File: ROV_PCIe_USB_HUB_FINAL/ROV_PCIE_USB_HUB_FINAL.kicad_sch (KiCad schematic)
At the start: 13 parts, among them J1 USB_A_Stacked, J2 USB_A_Stacked, J3 USB_A_Stacked, J4 USB_A_Stacked, U1 UPD720202K8-7x1-BAA, U2 USB2514B_Bi, U3 USB2514B_Bi, U4 USB2514B_Bi, U5 USB2514B_Bi

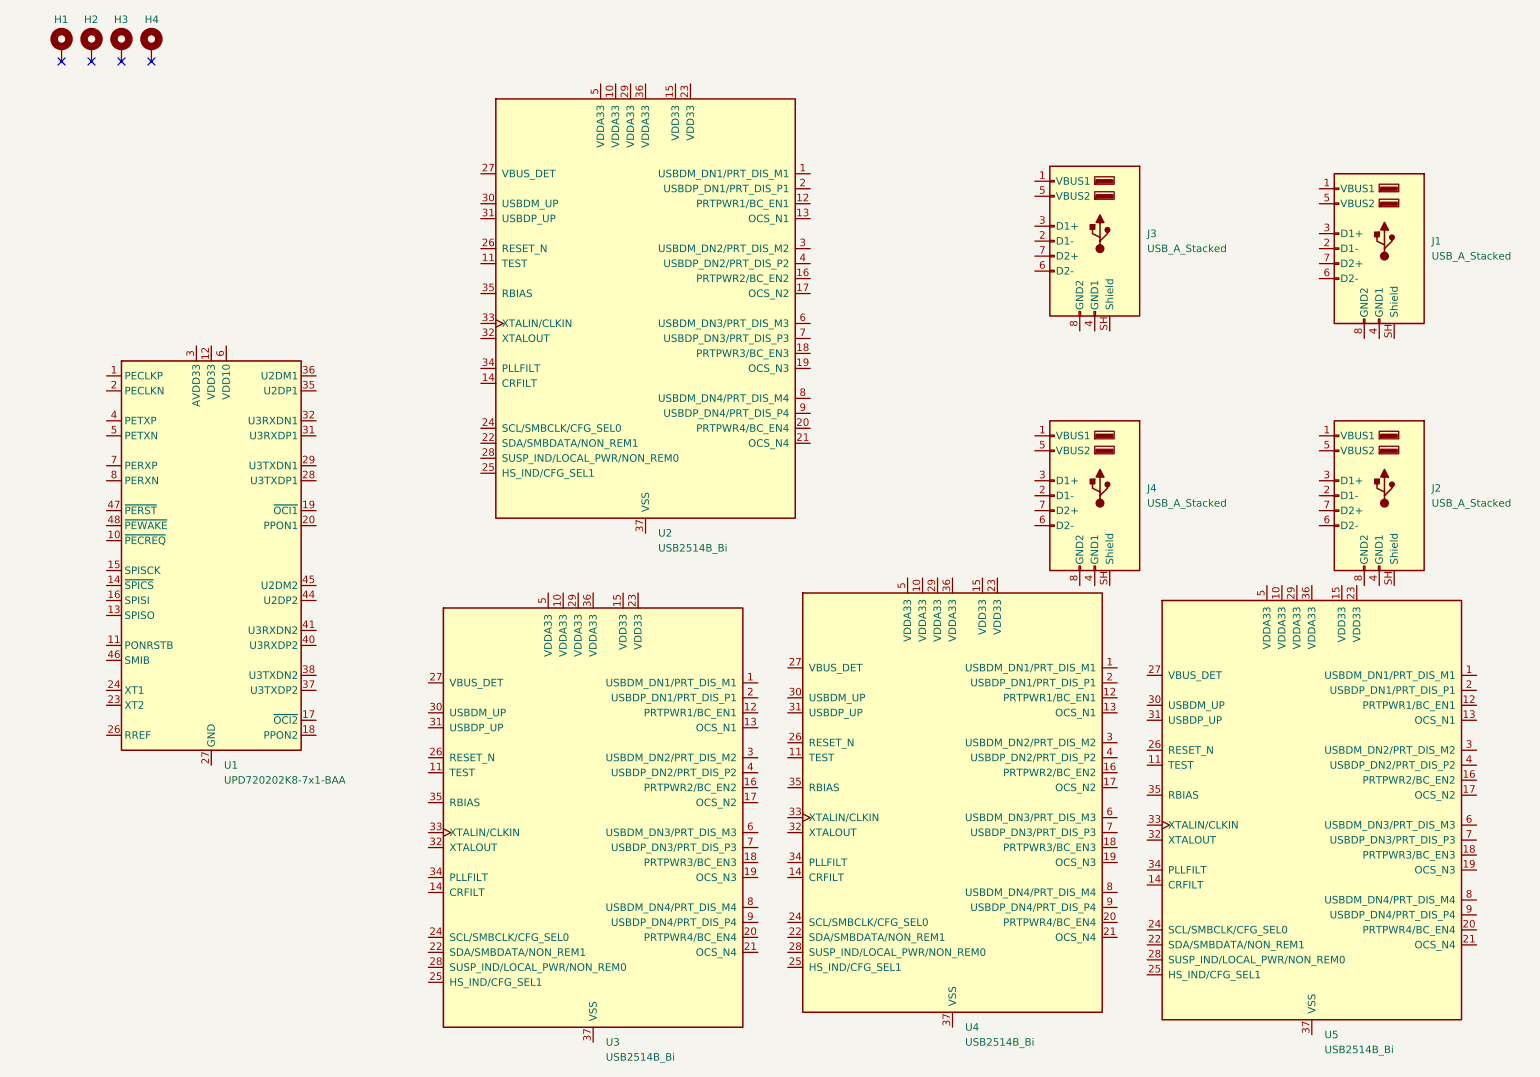
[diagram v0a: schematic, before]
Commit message: work
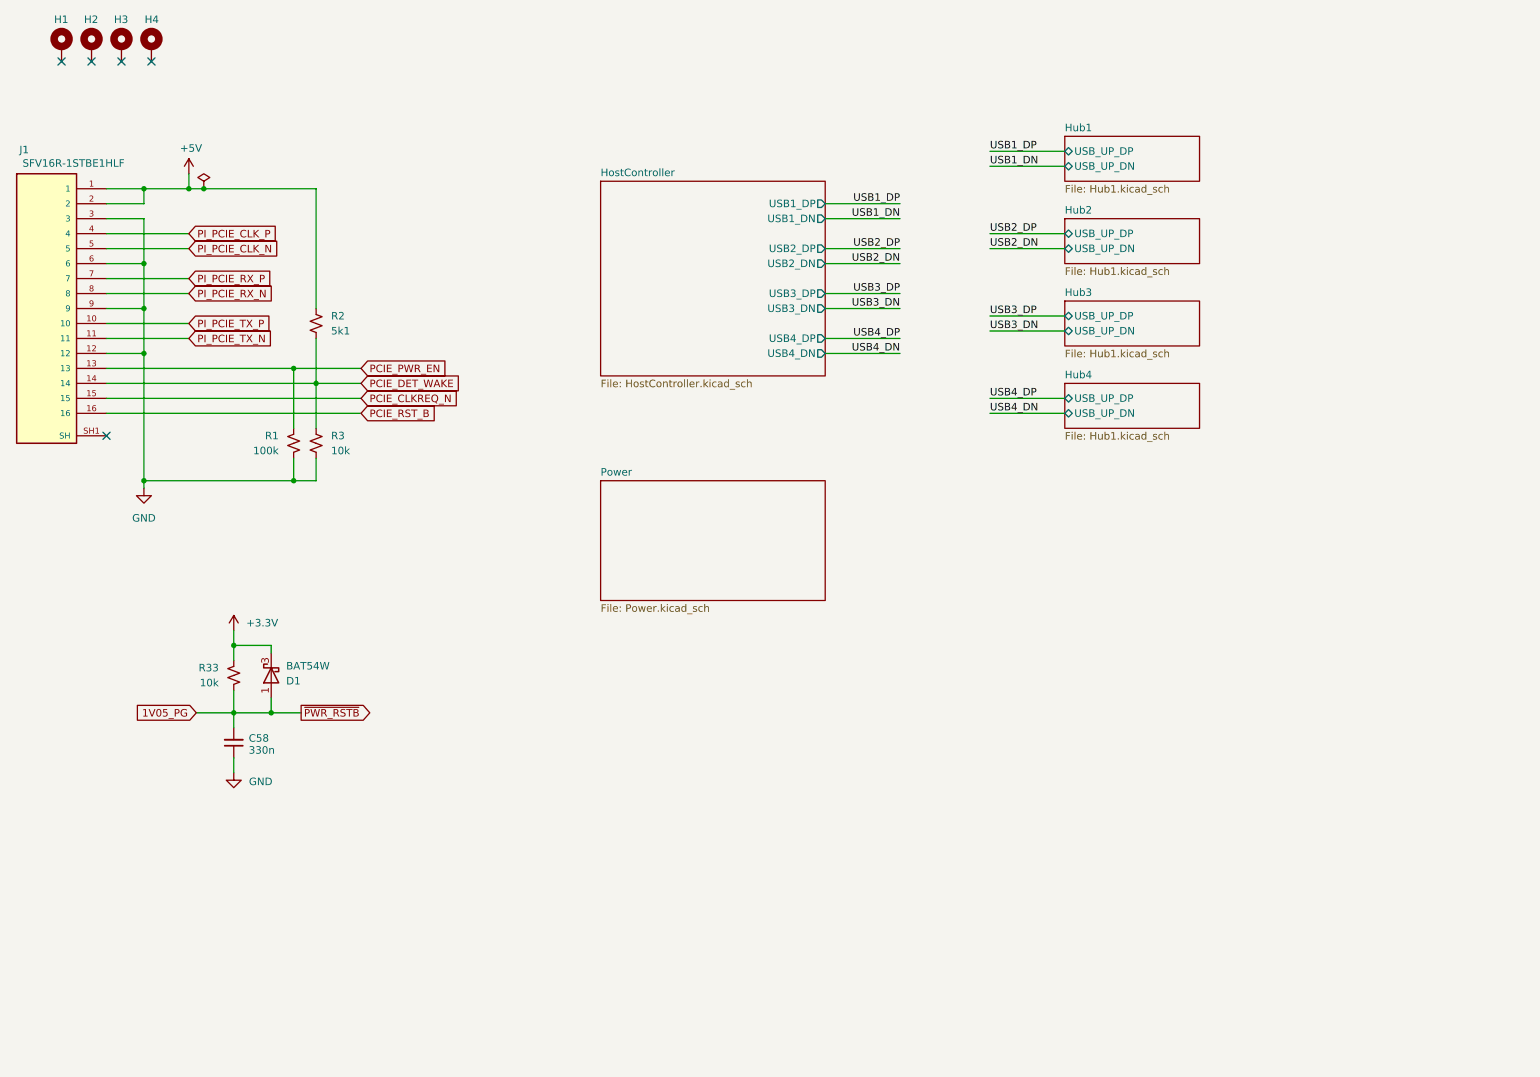
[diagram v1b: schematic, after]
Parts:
- removed J1, J2, J3, J4: USB_A_Stacked, Connector_USB:USB_A_CUI_UJ2-ADH-TH_Horizontal_Stacked, symbol Connector:USB_A_Stacked
- removed U1: UPD720202K8-7x1-BAA, Package_DFN_QFN:QFN-48-1EP_7x7mm_P0.5mm_EP5.7x5.7mm, symbol Interface_USB:UPD720202K8-7x1-BAA
- removed U2, U3, U4, U5: USB2514B_Bi, Package_DFN_QFN:QFN-36-1EP_6x6mm_P0.5mm_EP3.7x3.7mm, symbol Interface_USB:USB2514B_Bi
- added C58: 330n, Capacitor_SMD:C_0402_1005Metric, symbol Device:C_Small
- added D1: BAT54W, Package_TO_SOT_SMD:SOT-323_SC-70, symbol Diode:BAT54W
- added J1: SFV16R-1STBE1HLF, ROV_PCIe_USB_HUB:AMPHENOL_SFV16R-1STBE1HLF, symbol ROV_PCIe_USB_HUB:SFV16R-1STBE1HLF
- added R1: 100k, Resistor_SMD:R_0603_1608Metric, symbol Device:R_Small_US
- added R2: 5k1, Resistor_SMD:R_0603_1608Metric, symbol Device:R_Small_US
- added R3, R33: 10k, Resistor_SMD:R_0603_1608Metric, symbol Device:R_Small_US
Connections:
- new net: J1.SH1 (SH), J1.SH2 (SH)
- new net +3.3V: D1.3 (K), R33.1
- new net +5V: J1.1, J1.2, R2.1
- new net 1V05_PG: C58.2, D1.1 (A), R33.2
- new net GND: C58.1, J1.12, J1.3, J1.6, J1.9, R1.2, R3.2
- new net PCIE_CLKREQ_N: J1.15
- new net PCIE_DET_WAKE: J1.14, R2.2, R3.1
- new net PCIE_PWR_EN: J1.13, R1.1
- new net PCIE_RST_B: J1.16
- new net PI_PCIE_CLK_N: J1.5
- new net PI_PCIE_CLK_P: J1.4
- new net PI_PCIE_RX_N: J1.8
- new net PI_PCIE_RX_P: J1.7
- new net PI_PCIE_TX_N: J1.11
- new net PI_PCIE_TX_P: J1.10
- no-connect marks 4 -> 5
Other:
- added sheet HostController (HostController.kicad_sch)
- added sheet Hub1 (Hub1.kicad_sch)
- added sheet Hub2 (Hub1.kicad_sch)
- added sheet Hub3 (Hub1.kicad_sch)
- added sheet Hub4 (Hub1.kicad_sch)
- added sheet Power (Power.kicad_sch)
